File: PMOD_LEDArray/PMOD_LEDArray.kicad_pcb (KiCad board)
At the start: 2 copper layers, 130 parts, among them J1 Conn_02x06_Odd_Even, U1 GN1640

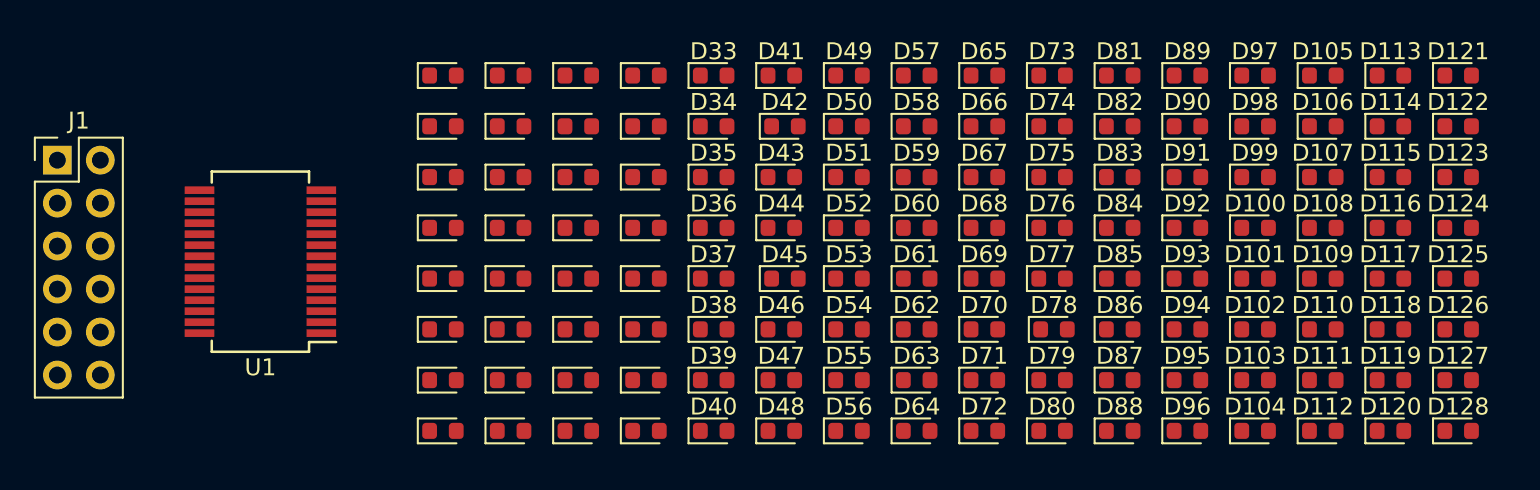
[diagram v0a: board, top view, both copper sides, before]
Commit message: Remove LED References and add board outline
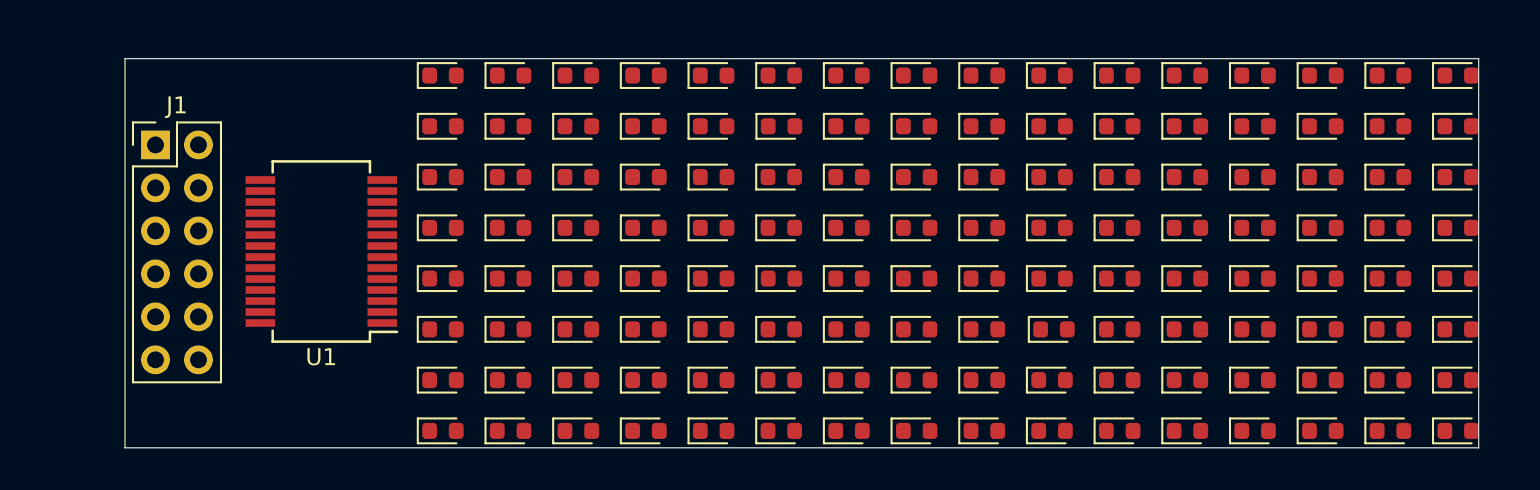
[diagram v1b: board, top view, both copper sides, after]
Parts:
- moved J1 5.87 mm to (106.8, 92.1)
- moved U1 3.65 mm to (116.6, 98.4)
- moved D42 0.20 mm to (143.8, 91.0)
- moved D45 0.20 mm to (143.8, 100.0)
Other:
- board outline added: 80 x 23 mm

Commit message: PCB initial layout complete
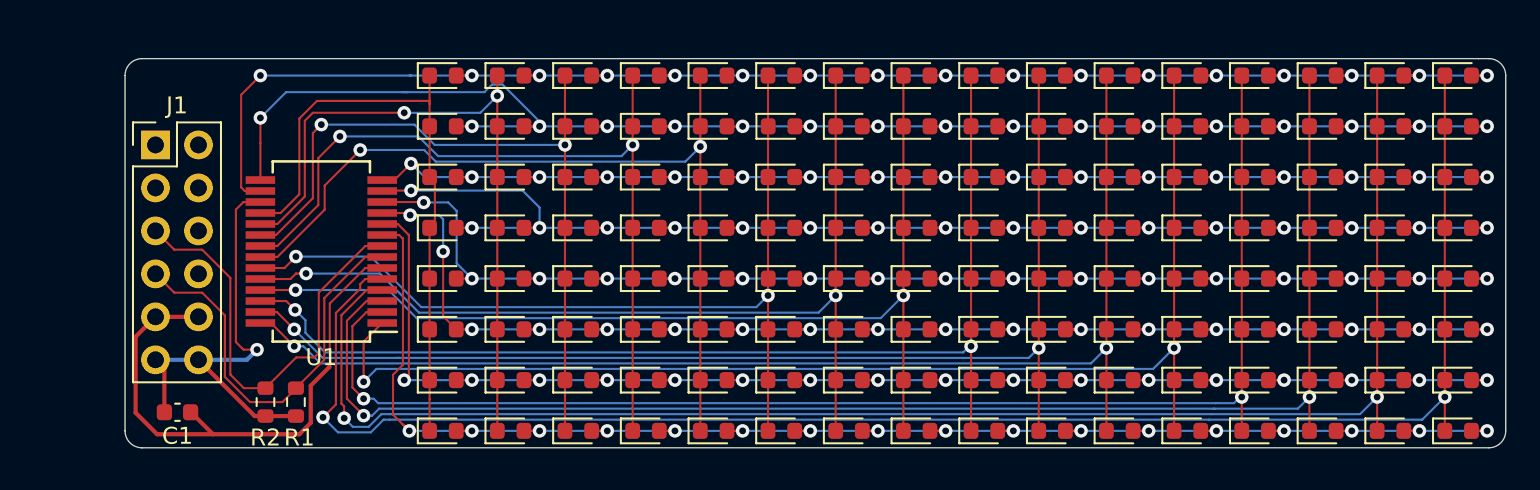
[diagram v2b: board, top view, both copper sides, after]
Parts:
- added C1: 100uF, Capacitor_SMD:C_0603_1608Metric, F.Cu at (108.1, 107.9)
- added R1: 10k, Resistor_SMD:R_0603_1608Metric, F.Cu at (115.1, 107.3)
- added R2: 10k, Resistor_SMD:R_0603_1608Metric, F.Cu at (113.3, 107.3)
- moved D78 0.11 mm to (159.8, 103.0)
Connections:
- U1 pad 5: /GRDI16 -> /GRID16
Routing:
- net /GRID16: track 0.00 -> 98.7 mm, vias 0 -> 2
- net /SEG7: track 0.00 -> 97.3 mm, vias 0 -> 17
- net /SEG8: track 0.00 -> 94.8 mm, vias 0 -> 17
- net /SEG1: track 0.00 -> 92.4 mm, vias 0 -> 17
- net /GRID15: track 0.00 -> 92.2 mm, vias 0 -> 2
- net /SEG2: track 0.00 -> 89.3 mm, vias 0 -> 17
- net /SEG3: track 0.00 -> 86.3 mm, vias 0 -> 18
- net /GRID14: track 0.00 -> 85.9 mm, vias 0 -> 2
- net /SEG5: track 0.00 -> 85.7 mm, vias 0 -> 17
- net /SEG4: track 0.00 -> 83.8 mm, vias 0 -> 17
- net /SEG6: track 0.00 -> 80.8 mm, vias 0 -> 17
- net /GRID13: track 0.00 -> 79.8 mm, vias 0 -> 2
- net /GRID12: track 0.00 -> 73.7 mm, vias 0 -> 2
- net /GRID11: track 0.00 -> 72.4 mm, vias 0 -> 2
- net /GRID10: track 0.00 -> 68.6 mm, vias 0 -> 2
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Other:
- board size 80 x 23 mm -> 81.6 x 23 mm
- rule trace_min: 0.2 -> 0.1
